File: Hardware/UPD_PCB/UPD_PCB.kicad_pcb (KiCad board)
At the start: 6 copper layers, 145 x 65 mm, 152 parts, among them IC1 STS30-DIS, J1 25A Fuse holder, J10 796739-2, J11 Conn_01x04, J12 Conn_01x02, J2 796739-2, J3 Conn_01x02, J4 1776119-2, J5 1776119-2, J6 1776119-2, J7 1776119-2, J8 1776119-2, J9 1776119-2, Q1 LMR51635XDDCR, Q2 LMR51635XDDCR, Q3 LMR51635XDDCR, Q4 LMR51635XDDCR, Q5 LMR51635XDDCR, Q6 LMR51635XDDCR, Q7 BSS84, U1 ACS711xEXLT-31AB, U2 INA219AxD, U3 INA219AxD, U4 INA219AxD, U5 INA219AxD, U6 INA219AxD, U7 INA219AxD

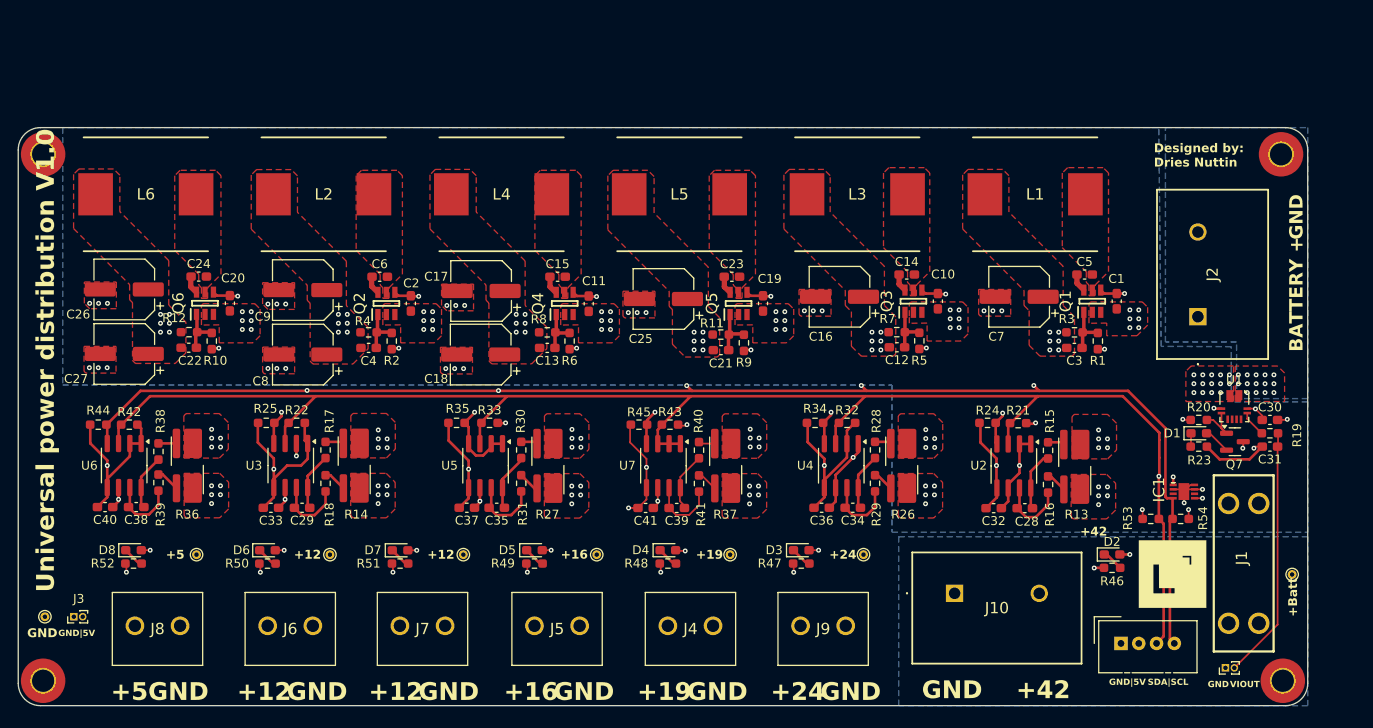
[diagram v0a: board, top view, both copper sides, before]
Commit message: Finalized pcb
Connector still needs to be changed
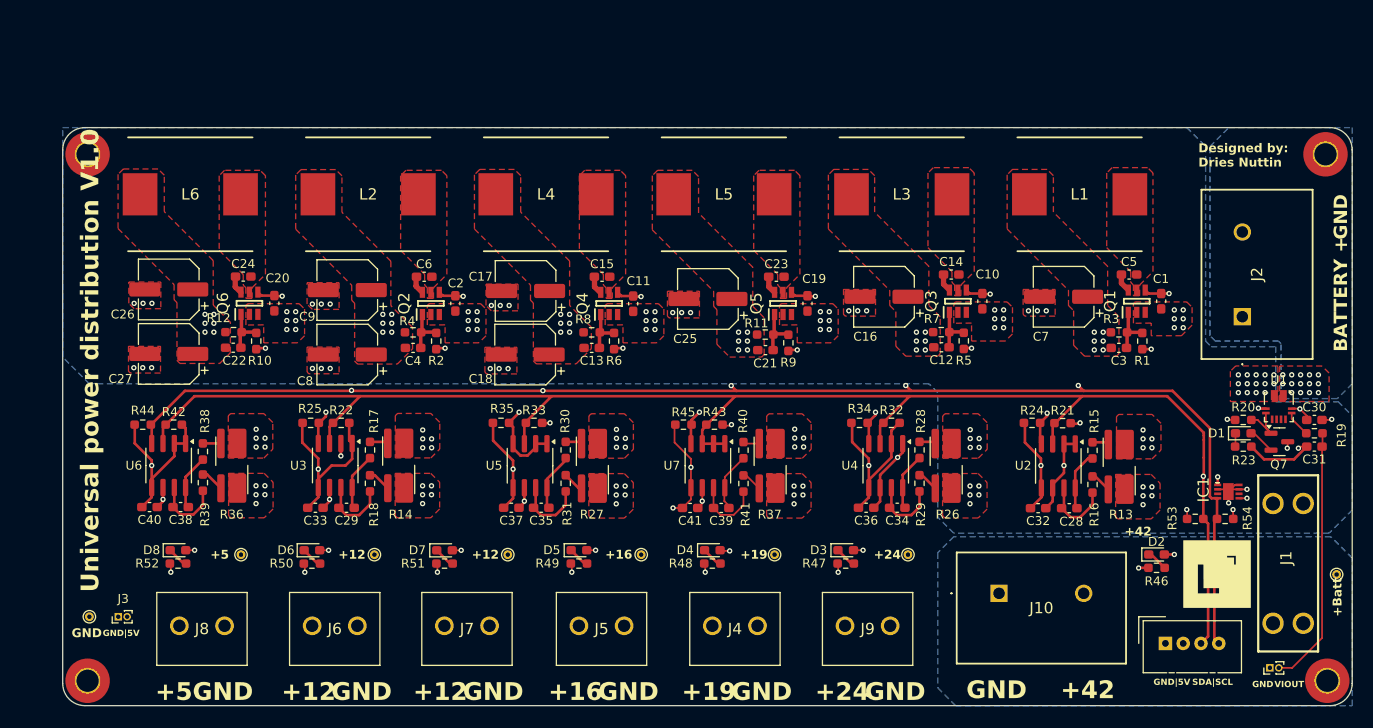
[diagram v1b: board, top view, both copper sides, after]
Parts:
- moved C29 5.00 mm to (131.9, 92.8)
- moved J6 5.00 mm to (128.1, 106.0)
- moved U3 5.00 mm to (130.6, 88.0)
- moved C1 5.00 mm to (223.5, 69.5)
- moved C10 5.00 mm to (203.4, 69.5)
- moved C11 5.00 mm to (164.2, 69.8)
- moved C12 5.00 mm to (198.8, 74.7)
- moved C13 5.00 mm to (159.5, 74.8)
- moved C14 5.00 mm to (199.9, 66.5)
- moved C15 5.00 mm to (160.6, 66.8)
- moved C16 5.00 mm to (192.3, 69.0)
- moved C17 5.00 mm to (152.1, 68.4)
- moved C18 5.00 mm to (152.0, 75.5)
- moved C19 5.00 mm to (183.8, 69.8)
- moved C2 5.00 mm to (144.2, 69.8)
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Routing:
- net GND: track 75.4 -> 76.6 mm
- net VIOUT: track 28.4 -> 29.3 mm
